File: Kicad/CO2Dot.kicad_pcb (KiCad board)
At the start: 4 copper layers, 25 x 40 mm, 31 parts, among them J2 USB_C_Receptacle, J4 Conn_01x02_Pin, J5 secondBoard, SW2 SW_Push, U1 AS7341-DLGT, U2 IP4234CZ6, U3 BME688, U5 AP7312-1833W6-7, U8 ESP8685, Y2 40MHz

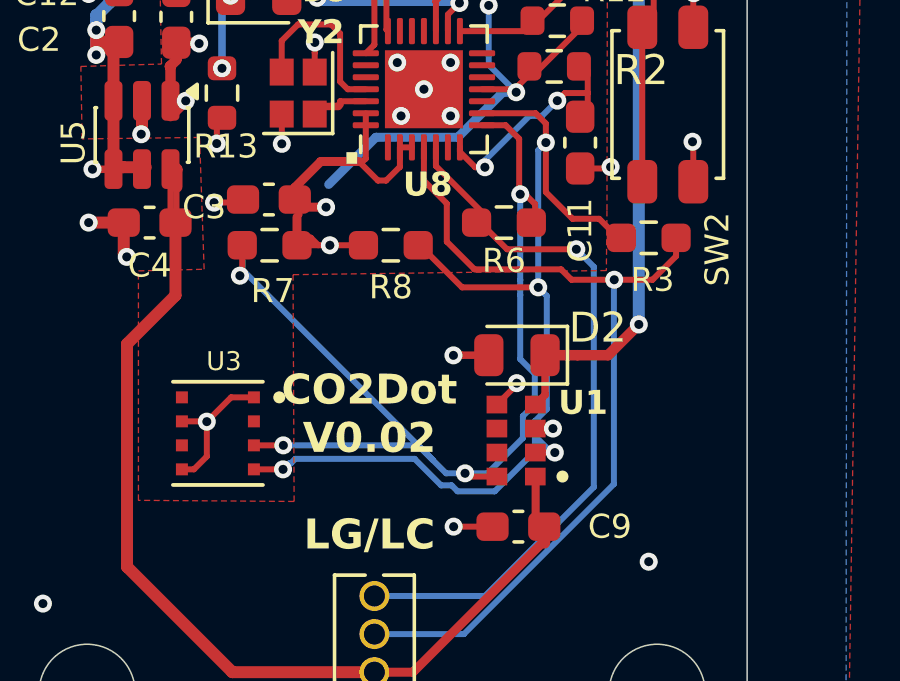
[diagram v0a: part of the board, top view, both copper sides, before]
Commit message: (kicad) fixed unconnected
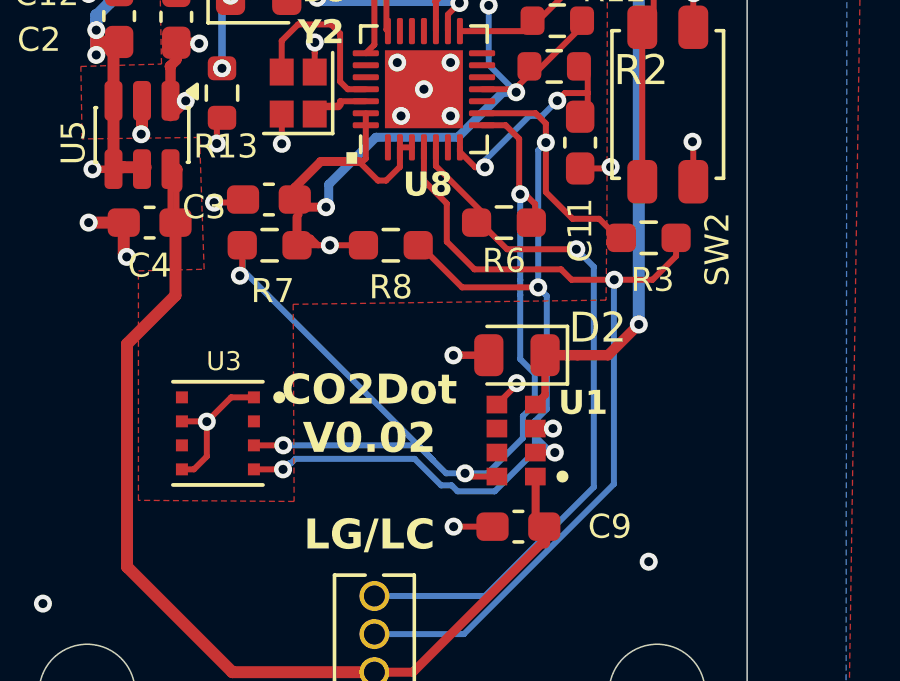
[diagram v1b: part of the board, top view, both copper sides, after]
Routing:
- net V+3V: track 37.0 -> 37.8 mm
